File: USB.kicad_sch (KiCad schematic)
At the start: 14 parts, among them J3 USB_C_Receptacle_USB2.0_16P, U2 CP2102N-Axx-xQFN24

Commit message: JLCPCB BOM and gerbers
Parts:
- D1: footprint Diode_SMD:D_SOD-323_HandSoldering -> Diode_SMD:D_SOD-123
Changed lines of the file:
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@@
 			)
 		)
-		(property "Footprint" "Diode_SMD:D_SOD-323_HandSoldering"
+		(property "Footprint" "Diode_SMD:D_SOD-123"
 			(at 67.31 35.56 0)
 			(effects

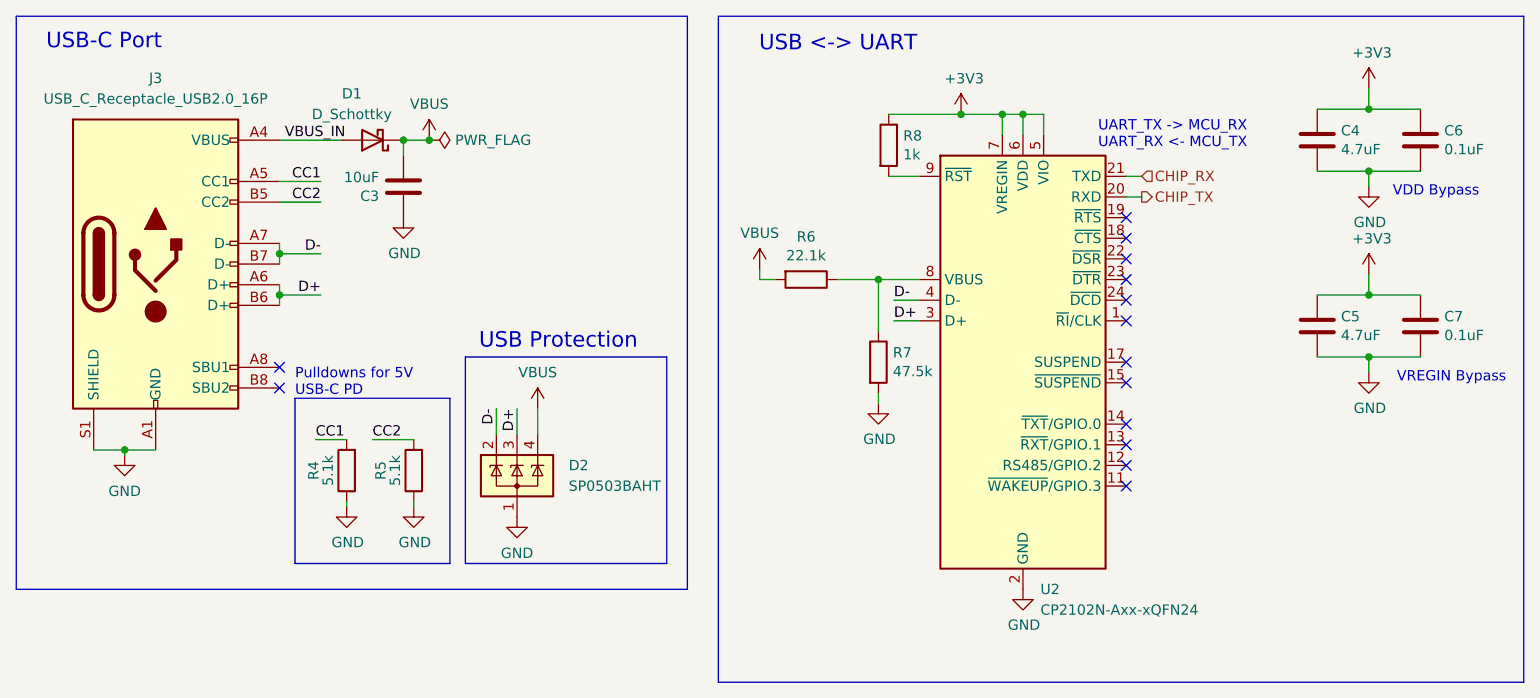
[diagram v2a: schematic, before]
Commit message: bom
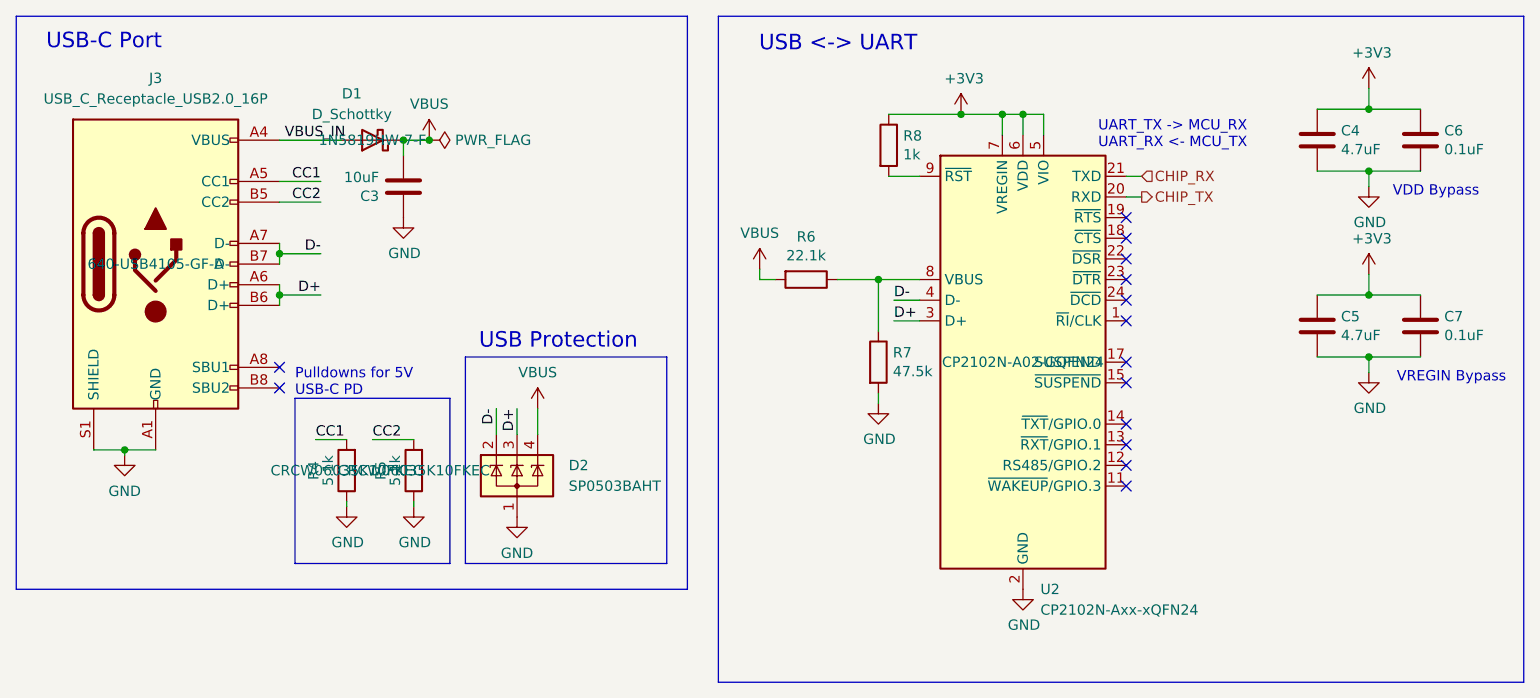
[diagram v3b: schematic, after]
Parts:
- C3: Mouser Part Number 581-22201C106KAT2A -> GRM21BR61H106KE43K
- C4, C5: Mouser Part Number 81-GRM219R6YA475KA3D -> 08055D475KAT4A
- C6, C7: Mouser Part Number 80-C0805C104M5R -> MLASH168SB7104KTNA01
- D1: Mouser Part Number (none) -> 1N5819HW-7-F
- J3: Mouser Part Number (none) -> 640-USB4105-GF-A
- R4, R5: Mouser Part Number (none) -> CRCW06035K10FKEC
- R6: Mouser Part Number 71-CRCW0805-22.1K-E3 -> CRCW060322K1FKEBC
- R7: Mouser Part Number 71-CRCW0805-47.5K-E3 -> CRCW060347K5FKEAHP
- R8: Mouser Part Number 71-CRCW08051K00FKEAC -> CRCW06031K00FKEI
- U2: Mouser Part Number (none) -> CP2102N-A02-GQFN24
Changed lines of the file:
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@@
 			)
 		)
-		(property "Mouser Part Number" "81-GRM219R6YA475KA3D"
+		(property "Mouser Part Number" "08055D475KAT4A"
 			(at 183.515 35.56 0)
 			(effects
@@
 			)
 		)
-		(property "Mouser Part Number" "80-C0805C104M5R"
+		(property "Mouser Part Number" "MLASH168SB7104KTNA01"
 			(at 196.215 35.56 0)
 			(effects
@@
 			)
 		)
+		(property "Mouser Part Number" "CRCW06035K10FKEC "
+			(at 64.135 76.2 0)
+			(effects
+				(font
+					(size 1.27 1.27)
+				)
+			)
+		)
 		(pin "1"
 		)
@@
 			)
 		)
-		(property "Mouser Part Number" "81-GRM219R6YA475KA3D"
+		(property "Mouser Part Number" "08055D475KAT4A"
 			(at 183.515 58.42 0)
 			(effects
@@
 			)
 		)
+		(property "Mouser Part Number" "CP2102N-A02-GQFN24"
+			(at 147.32 62.865 0)
+			(effects
+				(font
+					(size 1.27 1.27)
+				)
+			)
+		)
 		(pin "3"
 		)
@@
 			)
 		)
-		(property "Mouser Part Number" "71-CRCW08051K00FKEAC"
+		(property "Mouser Part Number" "CRCW06031K00FKEI "
 			(at 130.81 36.195 0)
 			(effects
@@
 			)
 		)
-		(property "Mouser Part Number" "581-22201C106KAT2A"
+		(property "Mouser Part Number" "GRM21BR61H106KE43K"
 			(at 71.12 41.275 0)
 			(effects
@@
 			)
 		)
-		(property "Mouser Part Number" "71-CRCW0805-22.1K-E3"
+		(property "Mouser Part Number" "CRCW060322K1FKEBC "
 			(at 120.65 52.705 0)
 			(effects
@@
 			)
 		)
-		(property "Mouser Part Number" "80-C0805C104M5R"
+		(property "Mouser Part Number" "MLASH168SB7104KTNA01"
 			(at 196.215 58.42 0)
 			(effects
@@
 			)
 		)
-		(property "Mouser Part Number" "71-CRCW0805-47.5K-E3"
+		(property "Mouser Part Number" "CRCW060347K5FKEAHP "
 			(at 129.54 62.865 0)
 			(effects
@@
 			)
 		)
+		(property "Mouser Part Number" "1N5819HW-7-F"
+			(at 67.31 35.56 0)
+			(effects
+				(font
+					(size 1.27 1.27)
+				)
+			)
+		)
 		(pin "2"
 		)
@@
 		)
 		(property "Vf" ""
+			(at 72.39 76.2 0)
+			(effects
+				(font
+					(size 1.27 1.27)
+				)
+			)
+		)
+		(property "Mouser Part Number" "CRCW06035K10FKEC "
 			(at 72.39 76.2 0)
 			(effects
@@
 			(at 40.64 50.8 0)
 			(effects
+				(font
+					(size 1.27 1.27)
+				)
+			)
+		)
+		(property "Mouser Part Number" "640-USB4105-GF-A"
+			(at 40.64 50.8 0)
+			(effects
